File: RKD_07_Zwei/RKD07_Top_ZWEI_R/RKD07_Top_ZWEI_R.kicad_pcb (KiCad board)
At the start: 2 copper layers, 242.9 x 102.4 mm, 58 parts, among them M5 Mark, M6 Mark, SW30 RotaryEncoder_Switch, SW51 SW_Push, SW52 SW_Push, SW53 SW_Push, SW54 SW_Push, SW55 SW_Push, SW56 SW_Push, SW57 SW_Push, SW58 SW_Push, SW59 SW_Push, SW61 SW_Push, SW62 SW_Push, SW63 SW_Push, SW64 SW_Push, SW66 SW_Push, SW67 SW_Push, SW68 SW_Push, SW69 SW_Push, SW70 SW_Push, SW71 SW_Push, SW72 SW_Push, SW73 SW_Push, SW74 SW_Push, SW75 SW_Push, SW76 SW_Push, SW77 SW_Push, SW78 SW_Push, SW79 SW_Push, SW80 SW_Push, SW81 SW_Push, SW82 SW_Push, SW83 SW_Push, SW84 SW_Push, SW85 SW_Push, SW86 SW_Push, SW87 SW_Push, SW88 SW_Push, SW89 SW_Push, SW90 SW_Push

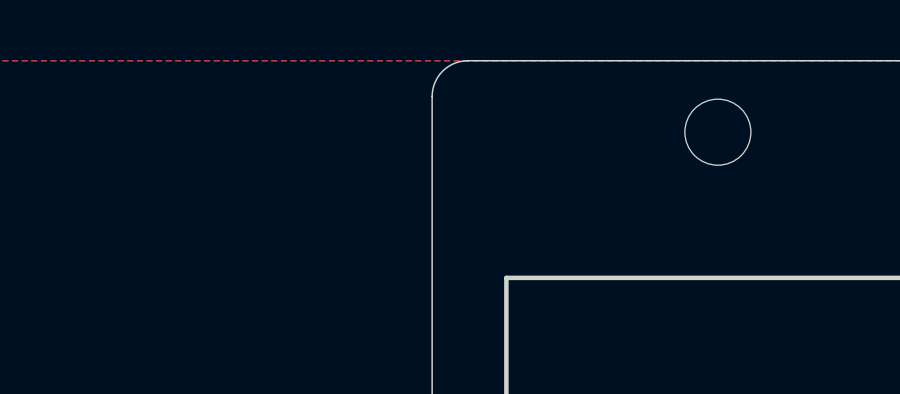
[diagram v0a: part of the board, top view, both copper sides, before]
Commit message: update
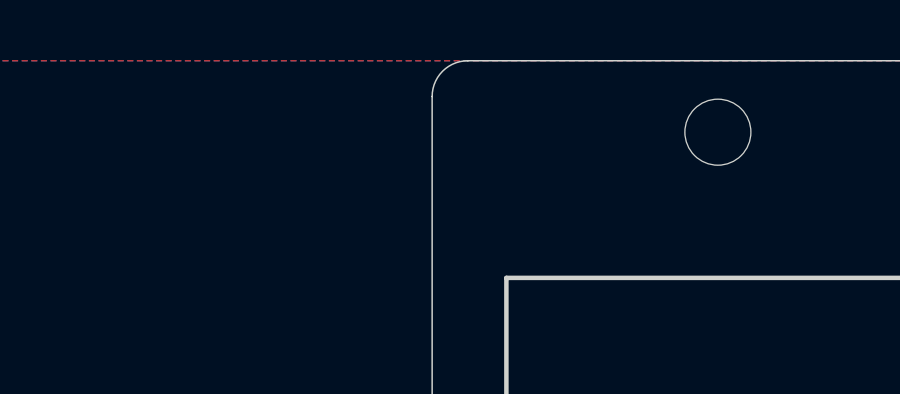
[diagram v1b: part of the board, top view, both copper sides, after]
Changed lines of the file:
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@@
 	(gr_arc
 		(start 242.887714 91.678553)
-		(mid 243.23641 90.836609)
+		(mid 243.236394 90.836604)
 		(end 244.078339 90.487928)
 		(stroke

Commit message: AddGuard
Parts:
- added Ref**: Val**, kbd_Hole:m2_Screw_Hole, F.Cu at (181.0, 92.9)
- added Ref**: Val**, kbd_Hole:m2_Screw_Hole, F.Cu at (238.1, 92.9)
- added Ref**: Val**, kbd_Hole:m2_Screw_Hole, F.Cu at (239.9, 102.4)
- added Ref**: Val**, kbd_Hole:m2_Screw_Hole, F.Cu at (239.9, 111.9)
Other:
- outline, holes or cut-outs redrawn
